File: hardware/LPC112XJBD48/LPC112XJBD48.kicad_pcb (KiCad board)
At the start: 2 copper layers, 23.6 x 23.5 mm, 28 parts, among them J1 Conn_02x09_Odd_Even, J2 Conn_02x09_Odd_Even, J3 JTAG_2X05, U1 LPC1125JBD48_303, Y1 12MHz

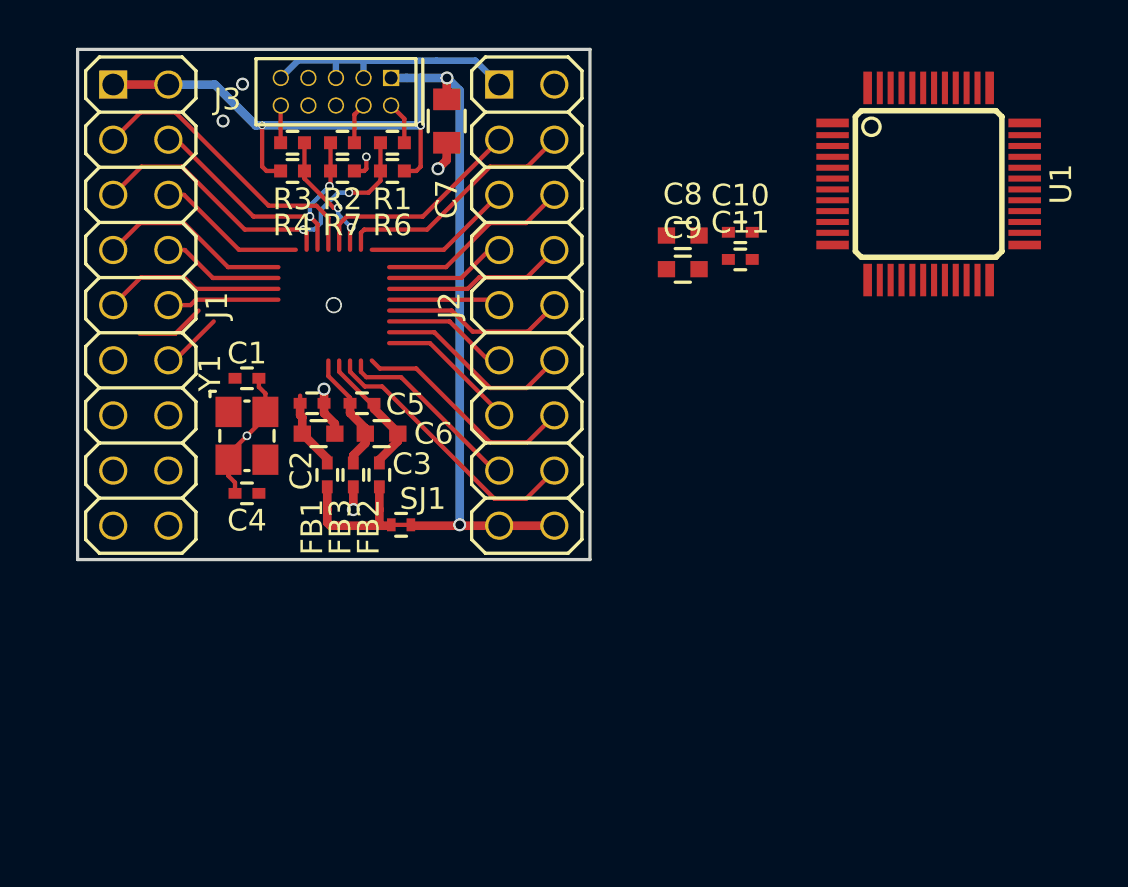
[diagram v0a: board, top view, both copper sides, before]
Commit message: further placement of components
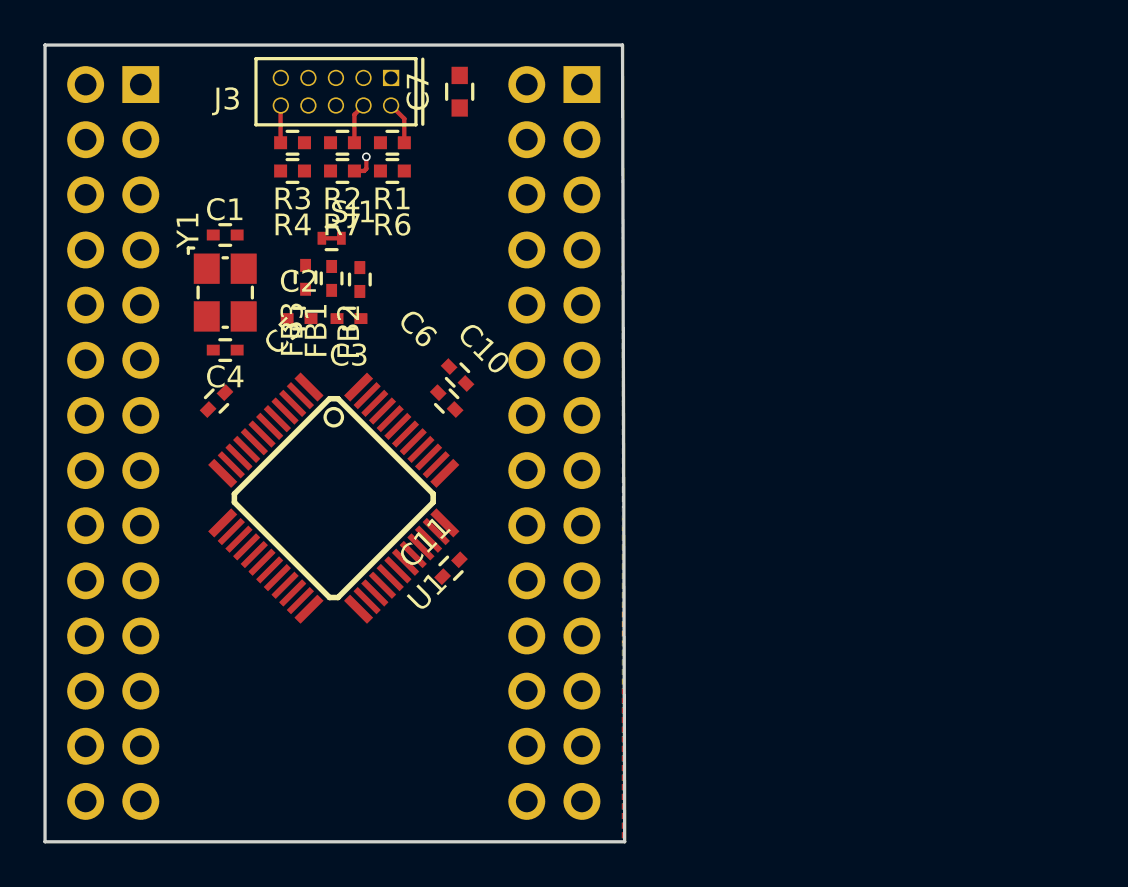
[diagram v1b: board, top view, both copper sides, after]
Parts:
- removed C8, C9: 1u, SquantorRcl:C_0603
- C2, C3: footprint SquantorRcl:C_0603 -> SquantorRcl:C_0402
- C7: footprint SquantorRcl:C_0805 -> SquantorRcl:C_0603
- J1, J2: value Conn_02x09_Odd_Even -> Conn_02x14_Odd_Even; footprint SquantorConnectors:Header-0254-2X09-H010 -> Connector_PinHeader_2.54mm:PinHeader_2x14_P2.54mm_Vertical; moved to B.Cu
- N2: value 20190310 -> 20190512
- moved U1 31.0 mm to (88.9, 115.6), turned to 225 degrees
- moved C11 19.5 mm to (94.3, 118.8), turned to 45 degrees
- moved C10 14.6 mm to (94.6, 109.9), turned to 315 degrees
- moved SJ1 13.6 mm to (88.8, 103.6)
- moved J2 10.5 mm to (100.3, 96.5), turned to 180 degrees
- moved J1 10.2 mm to (80.0, 96.5), turned to 180 degrees
- moved FB3 9.36 mm to (87.6, 105.4)
- moved FB1 9.05 mm to (88.8, 105.5)
- moved FB2 9.04 mm to (90.1, 105.5)
- moved Y1 6.68 mm to (83.9, 106.1)
- moved C1 6.68 mm to (83.9, 103.5)
- moved C4 6.68 mm to (83.9, 108.8)
- moved C3 5.51 mm to (89.6, 107.3)
- moved C2 5.38 mm to (87.3, 107.3)
- moved C5 4.40 mm to (83.5, 111.1), turned to 45 degrees
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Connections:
- J1 pad 10: (no net) -> /PIO2_7
- J1 pad 11: (no net) -> /PIO2_8
- J1 pad 12: (no net) -> VSS
- J1 pad 13: (no net) -> /PIO2_1
- J1 pad 14: (no net) -> /PIO0_3
- J1 pad 15: (no net) -> /PIO0_4
- J1 pad 16: (no net) -> /PIO0_5
- J1 pad 18: VSS -> /PIO1_9
- J1 pad 3: (no net) -> /PIO2_6
- J1 pad 4: (no net) -> /PIO2_0
- J1 pad 5: (no net) -> /RESET
- J1 pad 6: (no net) -> /PIO0_1
- J1 pad 7: /PIO0_10 -> VSS
- J1 pad 8: (no net) -> /PIO1_8
- J1 pad 9: (no net) -> /PIO0_2
- J2 pad 10: (no net) -> /PIO1_3
- J2 pad 11: (no net) -> /PIO2_3
- J2 pad 12: (no net) -> VSS
- J2 pad 13: (no net) -> /PIO3_0
- J2 pad 14: (no net) -> /PIO1_2
- J2 pad 15: (no net) -> /PIO1_1
- J2 pad 16: (no net) -> /PIO1_0
- J2 pad 17: VDD -> VSS
- J2 pad 18: VDD -> /PIO0_11
- J2 pad 3: (no net) -> /PIO3_3
- J2 pad 4: (no net) -> /PIO1_7
- J2 pad 5: (no net) -> /PIO1_6
- J2 pad 6: (no net) -> /PIO1_5
- J2 pad 7: (no net) -> VSS
- J2 pad 8: (no net) -> /PIO1_11
- J2 pad 9: (no net) -> /PIO1_4
- U1 pad 1: (no net) -> /PIO2_6
- U1 pad 10: (no net) -> /PIO0_2
- U1 pad 11: (no net) -> /PIO2_7
- U1 pad 12: (no net) -> /PIO2_8
- U1 pad 13: (no net) -> /PIO2_1
- U1 pad 14: (no net) -> /PIO0_3
- U1 pad 15: (no net) -> /PIO0_4
- U1 pad 16: (no net) -> /PIO0_5
- U1 pad 17: (no net) -> /PIO1_9
- U1 pad 18: (no net) -> /PIO3_4
- U1 pad 19: (no net) -> /PIO2_4
- U1 pad 2: (no net) -> /PIO2_0
- U1 pad 20: (no net) -> /PIO2_5
- U1 pad 21: (no net) -> /PIO3_5
- U1 pad 22: (no net) -> /PIO0_6
- U1 pad 23: (no net) -> /PIO0_7
- U1 pad 24: (no net) -> /PIO2_9
- U1 pad 25: (no net) -> /PIO2_2
- U1 pad 26: (no net) -> /PIO0_8
- U1 pad 27: (no net) -> /PIO0_9
- U1 pad 29: (no net) -> /PIO1_10
- U1 pad 30: (no net) -> /PIO0_11
- U1 pad 31: (no net) -> /PIO1_0
- U1 pad 32: (no net) -> /PIO1_1
- U1 pad 35: (no net) -> /PIO1_2
- U1 pad 36: (no net) -> /PIO3_0
- U1 pad 37: (no net) -> /PIO2_3
- U1 pad 39: (no net) -> /PIO1_4
- U1 pad 4: (no net) -> /PIO0_1
- U1 pad 42: (no net) -> /PIO1_11
- U1 pad 45: (no net) -> /PIO1_5
- U1 pad 46: (no net) -> /PIO1_6
- U1 pad 47: (no net) -> /PIO1_7
- U1 pad 48: (no net) -> /PIO3_3
- U1 pad 9: (no net) -> /PIO1_8
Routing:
- net (no net): track 165.2 -> 0.00 mm
- net VDD: track 53.8 -> 0.00 mm, vias 4 -> 0
- net VSS: track 24.8 -> 1.14 mm, vias 7 -> 1
- net /PIO0_2: track 18.1 -> 0.00 mm, vias 2 -> 0
- net /PIO0_3: track 13.5 -> 0.00 mm, vias 2 -> 0
- net /PIO0_10: track 8.96 -> 0.00 mm
- net Net-(FB1-Pad2): track 6.46 -> 0.00 mm
- net Net-(C11-Pad1): track 6.28 -> 0.00 mm, vias 1 -> 0
- net /RESET: track 6.06 -> 0.00 mm, vias 2 -> 0
- net Net-(C11-Pad2): track 5.65 -> 0.00 mm
- net Net-(C10-Pad1): track 3.62 -> 0.00 mm
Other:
- board size 23.6 x 23.5 mm -> 26.7 x 36.7 mm
